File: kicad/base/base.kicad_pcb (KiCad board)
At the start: 2 copper layers, 63 x 50 mm, 23 parts, among them J1 TO ARM, Q1 MMBT3904, Q2 MMBT3904, Q3 MMBT3904, SW2 SW_SPST_LED_RGB, U1 Seeeduiono_Xiao, U2 NC7SB3257P6X, U3 AS5600

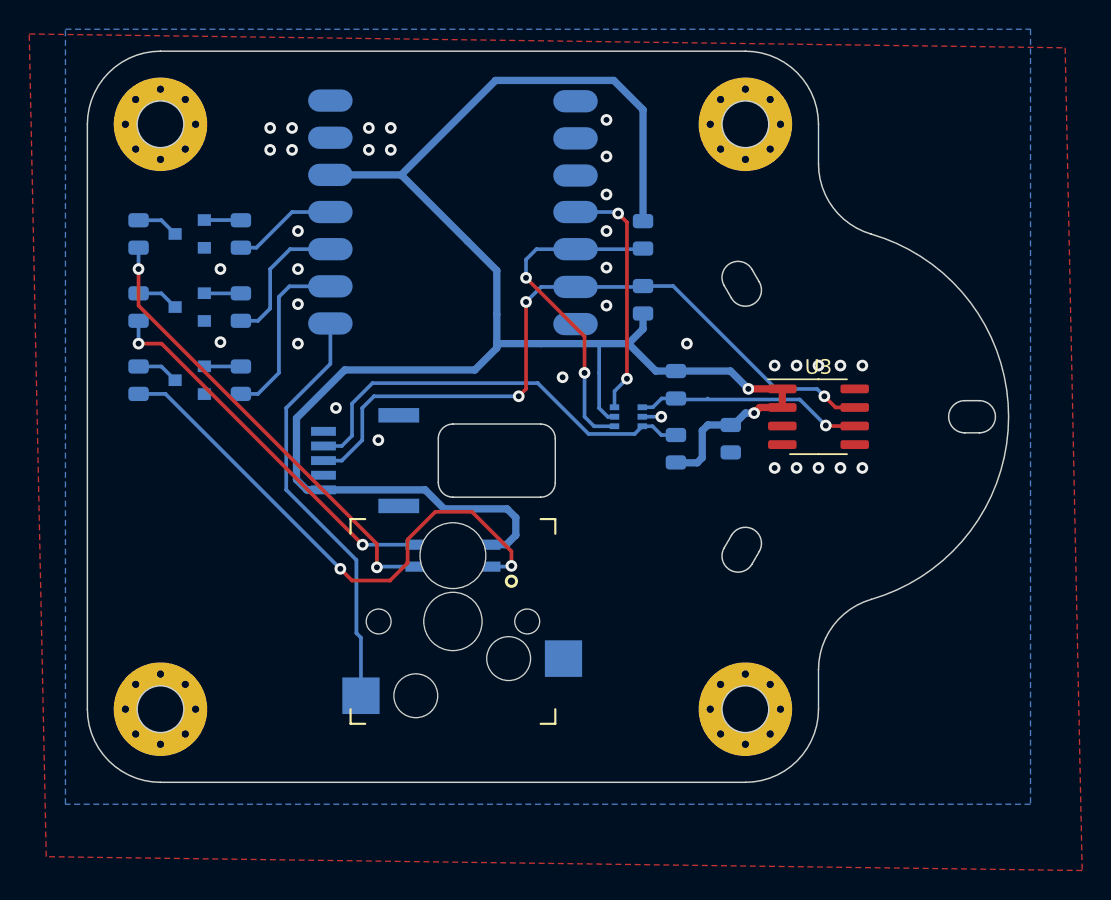
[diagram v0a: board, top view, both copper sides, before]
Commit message: something
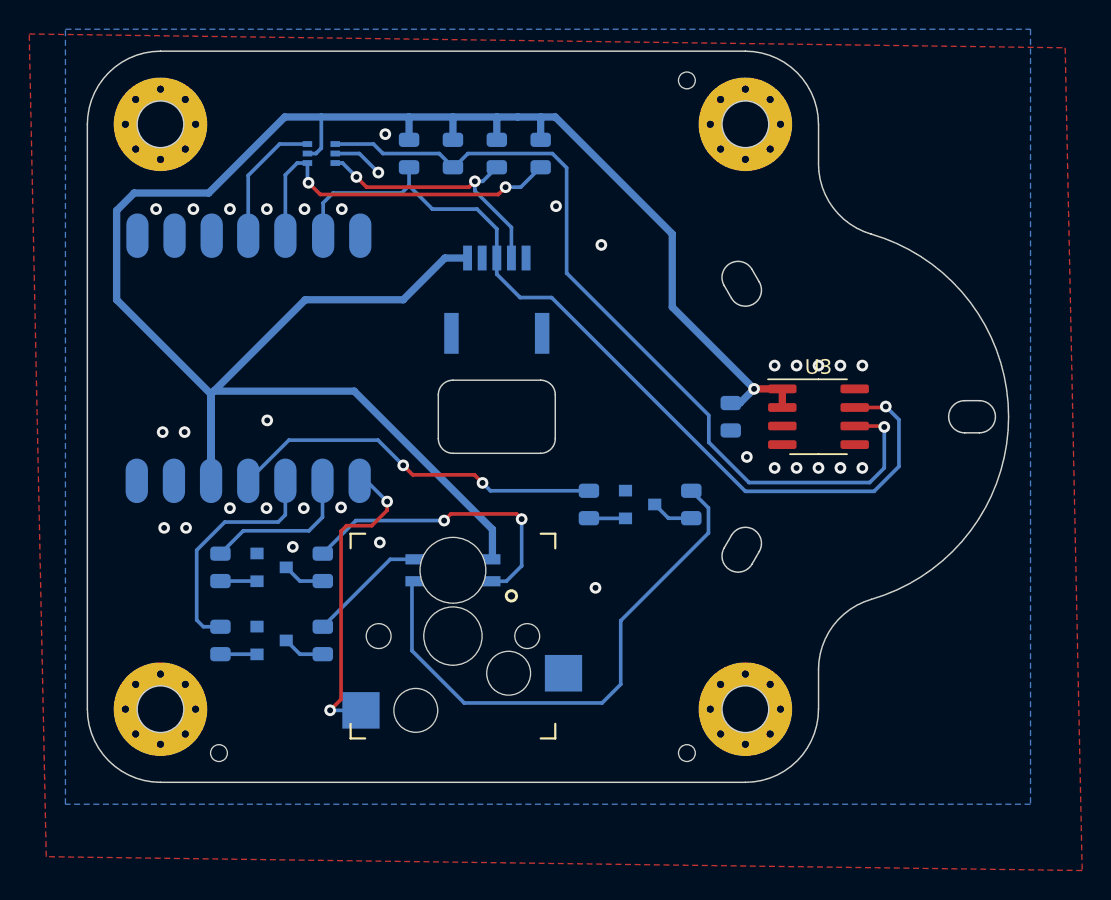
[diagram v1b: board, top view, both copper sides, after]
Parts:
- added REF**: JLCPCB Tooling Hole, base:JLCPCB Tooling Hole, F.Cu at (158.0, 73.0)
- added REF**: JLCPCB Tooling Hole, base:JLCPCB Tooling Hole, F.Cu at (126.0, 119.0)
- added REF**: JLCPCB Tooling Hole, base:JLCPCB Tooling Hole, F.Cu at (158.0, 119.0)
- R5: value 65R -> 68R
- moved R6 42.1 mm to (158.3, 102.0), turned to 270 degrees
- moved Q1 35.9 mm to (154.8, 102.0), turned to 0 degrees
- moved R8 30.1 mm to (151.3, 102.0), turned to 90 degrees
- moved U2 27.7 mm to (133.0, 78.0)
- moved R5 26.0 mm to (133.1, 111.3), turned to 270 degrees
- moved R3 23.6 mm to (145.0, 78.0), turned to 270 degrees
- moved Q2 23.5 mm to (129.6, 111.3), turned to 0 degrees
- moved R9 22.8 mm to (126.1, 111.3), turned to 90 degrees
- moved R2 22.0 mm to (142.0, 78.0)
- moved R1 18.9 mm to (139.0, 78.0), turned to 270 degrees
- moved R7 18.0 mm to (133.1, 106.3), turned to 270 degrees
- moved U1 17.2 mm to (128.0, 92.0), turned to 270 degrees
- moved J1 14.2 mm to (145.0, 88.0), turned to 180 degrees
- moved Q3 14.0 mm to (129.6, 106.3), turned to 0 degrees
- moved R10 12.9 mm to (126.1, 106.3), turned to 90 degrees
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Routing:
- net SDA1: track 15.6 -> 58.5 mm
- net G_CONT: track 7.13 -> 25.9 mm, vias 0 -> 2
- net Net-(R5-Pad1): track 26.3 -> 8.06 mm, vias 2 -> 0
- net +3V3: track 127.4 -> 145.1 mm, vias 2 -> 1
- net Net-(R7-Pad1): track 37.3 -> 20.6 mm
- net SCL: track 49.5 -> 61.2 mm, vias 3 -> 1
- net SDA2: track 29.1 -> 18.6 mm, vias 0 -> 2
- net SEL: track 16.8 -> 9.06 mm, vias 2 -> 0
- net EN_SW: track 28.8 -> 21.5 mm, vias 0 -> 2
- net R_CONT: track 9.73 -> 16.0 mm
- net Net-(R6-Pad1): track 31.4 -> 37.3 mm, vias 2 -> 0
- net GND: track 1.30 -> 3.49 mm, vias 35 -> 33
- net B_CONT: track 12.2 -> 10.5 mm
- net SDA: track 23.5 -> 24.4 mm
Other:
- outline, holes or cut-outs redrawn
